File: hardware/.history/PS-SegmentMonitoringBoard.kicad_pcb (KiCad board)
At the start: 4 copper layers, 75 x 80.3 mm, 124 parts, among them IC1 BQ79616PAPR, J1 voltTapsConn, J2 highSideConn, J3 lowSideConn, J4 thermsConn, Q1 ZXTN4004KTC

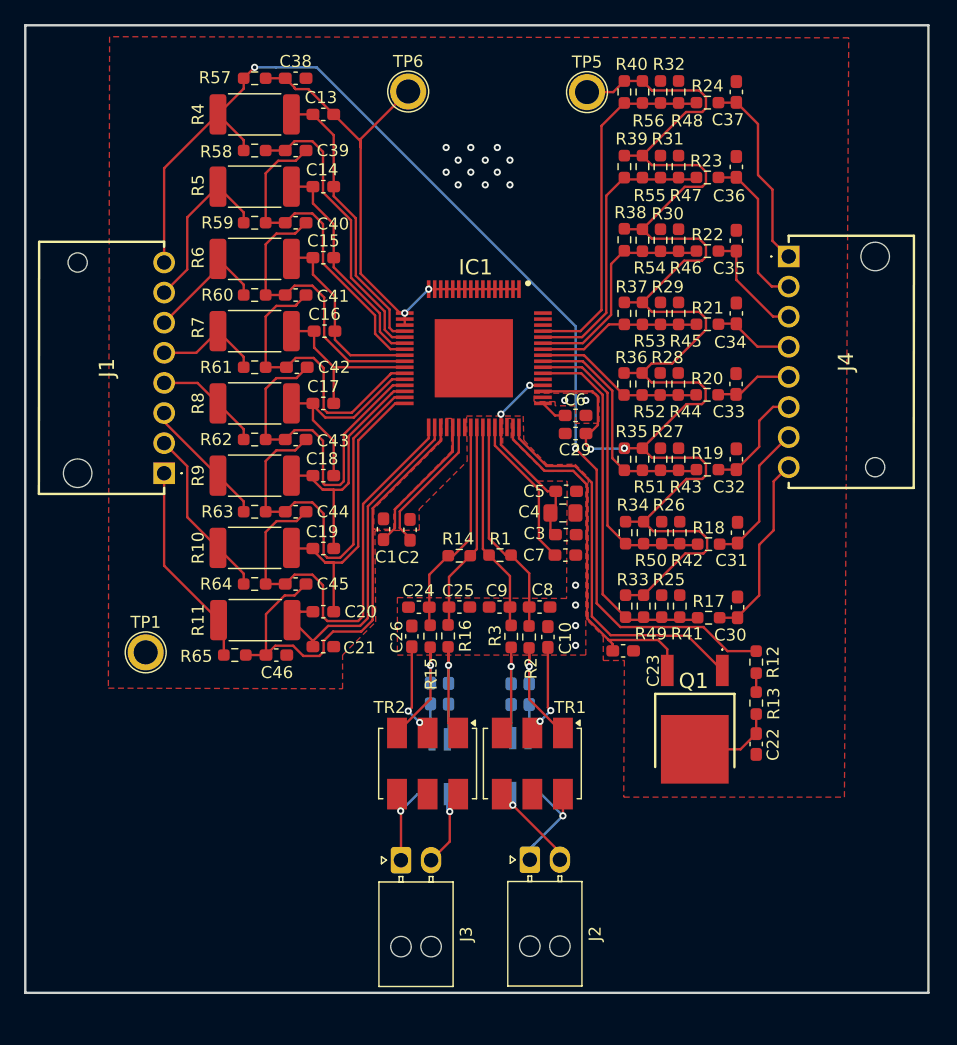
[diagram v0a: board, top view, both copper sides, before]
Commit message: layout fp updates, CB trace increases, n more
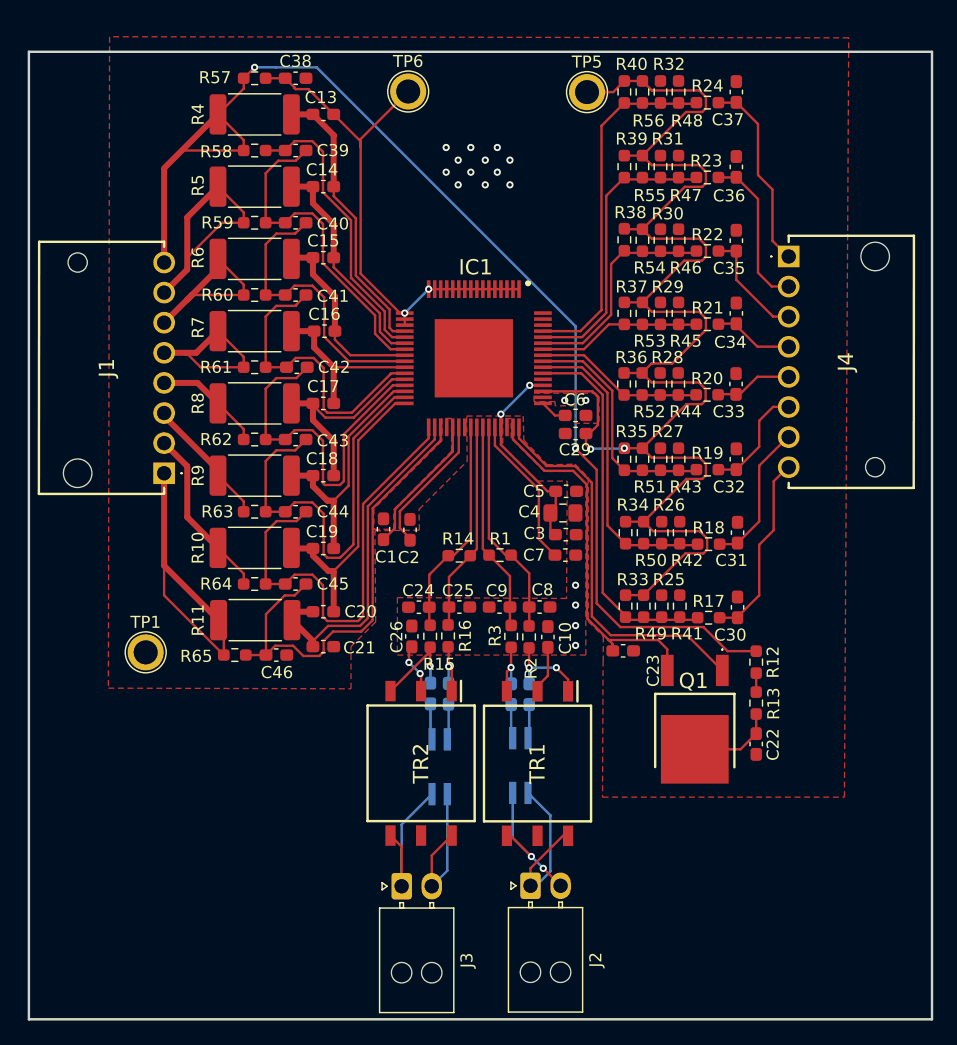
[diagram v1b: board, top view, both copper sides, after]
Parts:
- TR1, TR2: footprint RF_Mini-Circuits:Mini-Circuits_CD636_H4.11mm -> Custom-Footprints:SOP254P1270X685-6N
- moved J2 2.17 mm to (124.7, 132.3)
- moved J3 2.17 mm to (114.0, 132.3)
- moved TR2 0.54 mm to (113.1, 122.1)
- moved TR1 0.43 mm to (122.8, 122.2)
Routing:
- net /Cell_Balancing/V0: track 18.1 -> 35.2 mm
- net /Cell_Balancing/V6: track 14.5 -> 21.4 mm
- net /Cell_Balancing/V7: track 99.1 -> 105.5 mm
- net /lowSideIsolation/preIsolationCOMHN: track 10.5 -> 5.19 mm
- net /Cell_Balancing/V4: track 9.10 -> 14.4 mm
- net /lowSideIsolation/isolatedCOMLN: track 7.95 -> 13.1 mm, vias 1 -> 0
- net /Cell_Balancing/V5: track 11.0 -> 15.9 mm
- net /highSideIsolation/preIsolationCOMHN: track 9.67 -> 5.14 mm
- net /lowSideIsolation/isolatedCOMLP: track 8.81 -> 13.3 mm, vias 1 -> 0
- net /highSideIsolation/isolatedCOMHP: track 10.9 -> 15.1 mm, vias 1 -> 0
- net Net-(C26-Pad2): track 8.12 -> 4.19 mm
- net Net-(C10-Pad2): track 7.87 -> 4.00 mm, vias 2 -> 0
- net /highSideIsolation/preIsolationCOMHP: track 11.2 -> 7.61 mm, vias 1 -> 2
- net /highSideIsolation/isolatedCOMHN: track 8.67 -> 12.1 mm, vias 1 -> 2
- net /lowSideIsolation/preIsolationCOMHP: track 11.2 -> 8.00 mm
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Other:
- board size 75 x 80.3 mm -> 75 x 80.4 mm
